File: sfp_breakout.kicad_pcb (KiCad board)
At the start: 2 copper layers, 62.5 x 64 mm, 19 parts, among them J1 TD-, J2 TD+, J3 RD+, J4 RD-, J5 Conn, U1 SFP

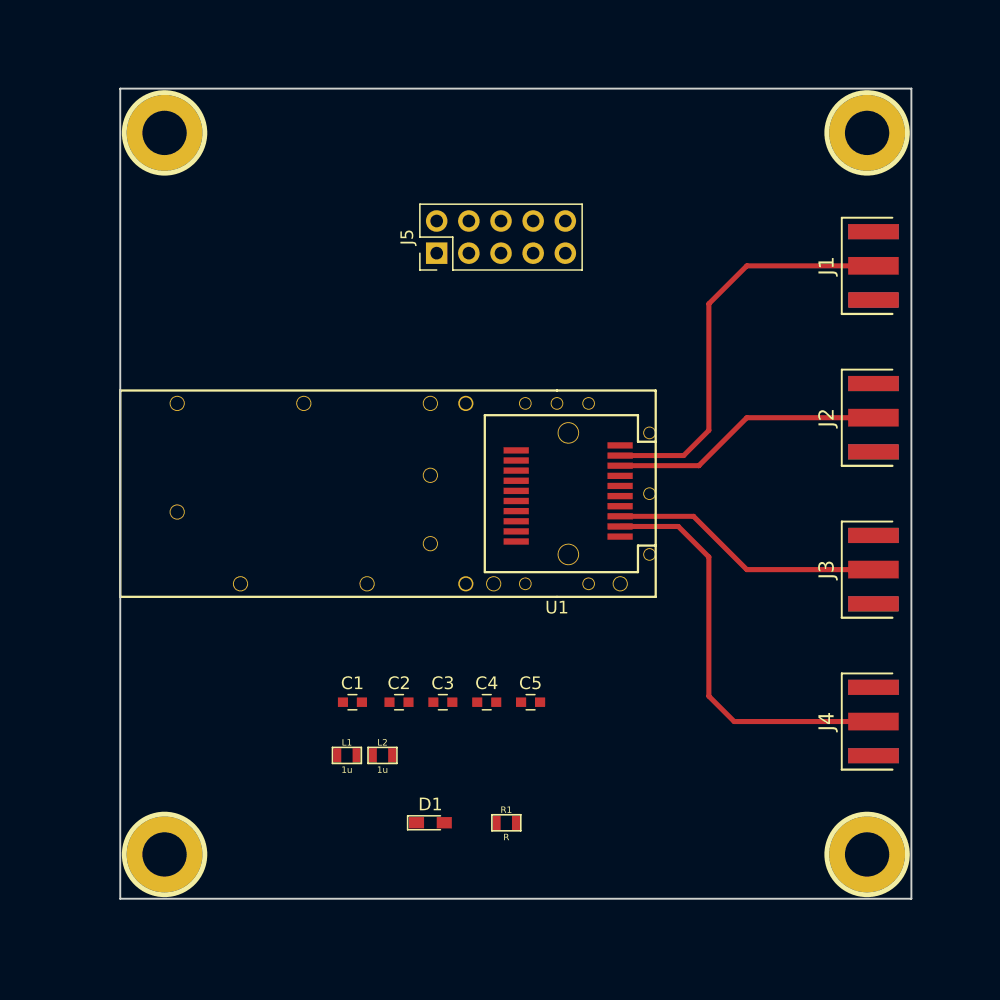
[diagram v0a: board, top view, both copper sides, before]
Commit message: Did some layout and routing
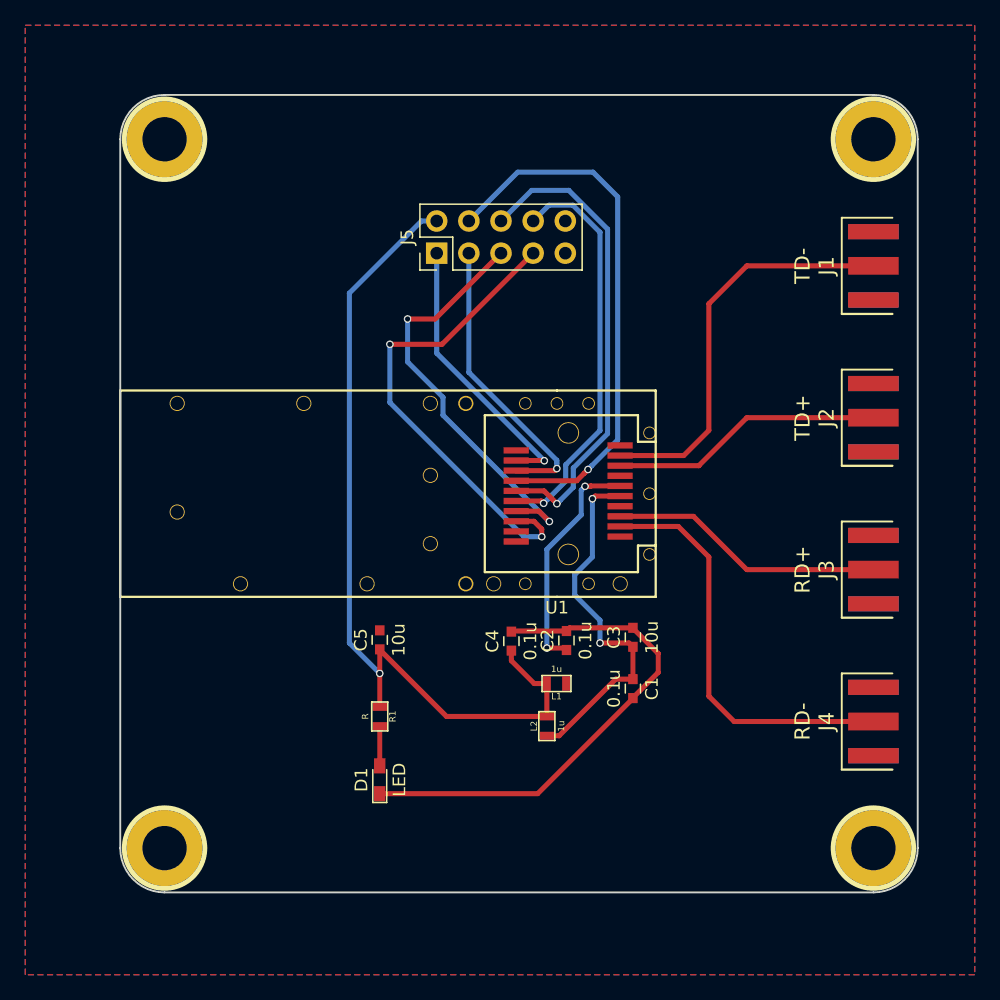
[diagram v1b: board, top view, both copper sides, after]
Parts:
- moved C1 22.2 mm to (98.0, 87.4), turned to 270 degrees
- moved L1 17.5 mm to (92.0, 87.0), turned to 180 degrees
- moved C3 15.9 mm to (98.0, 83.3), turned to 90 degrees
- moved C2 14.1 mm to (92.8, 83.6), turned to 90 degrees
- moved L2 13.2 mm to (91.2, 90.4), turned to 90 degrees
- moved R1 13.1 mm to (78.0, 89.6), turned to 270 degrees
- moved C5 12.9 mm to (78.0, 83.5), turned to 90 degrees
- moved D1 5.25 mm to (78.0, 94.6), turned to 90 degrees
- moved C4 5.20 mm to (88.4, 83.7), turned to 90 degrees
- moved h? 0.71 mm to (117.0, 44.0)
- moved h? 0.71 mm to (117.0, 100.0)
- moved h? 0.50 mm to (61.0, 100.0)
- moved h? 0.50 mm to (61.0, 44.0)
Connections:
- U1 pad : (no net) -> GND
- U1 pad  : (no net) -> GND
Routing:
- net +3V3: track 0.00 -> 67.2 mm, vias 0 -> 1
- net Def-2: track 0.00 -> 42.7 mm, vias 0 -> 1
- net GND: track 0.00 -> 40.1 mm
- net LOS: track 0.00 -> 38.2 mm, vias 0 -> 2
- net Def-1: track 0.00 -> 37.7 mm, vias 0 -> 1
- net Rate-Sel: track 0.00 -> 33.1 mm, vias 0 -> 2
- net Def-0: track 0.00 -> 32.2 mm, vias 0 -> 1
- net Net-(C1-Pad1): track 0.00 -> 29.0 mm, vias 0 -> 2
- net TxDisable: track 0.00 -> 23.2 mm, vias 0 -> 1
- net TxFault: track 0.00 -> 22.1 mm, vias 0 -> 1
- net Net-(C2-Pad1): track 0.00 -> 18.4 mm, vias 0 -> 2
- net Net-(D1-Pad2): track 0.00 -> 3.14 mm
- added copper zone on B.Cu, net GND
- added copper zone on F.Cu, net GND
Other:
- board size 62.5 x 64 mm -> 63 x 63 mm
